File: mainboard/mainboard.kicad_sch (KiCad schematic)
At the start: 54 parts, among them J1 Servo, J2 Buzzer, J4 Button Interface, J5 Power, J6 Release Button, J7 Extra Pins, Q1 BSS138, SW1 SW_Push, U1 RP2040, U2 W25Q128JVS, U3 RV-3028-C7, U4 ITR9608-F, Y1 Crystal_ABM8

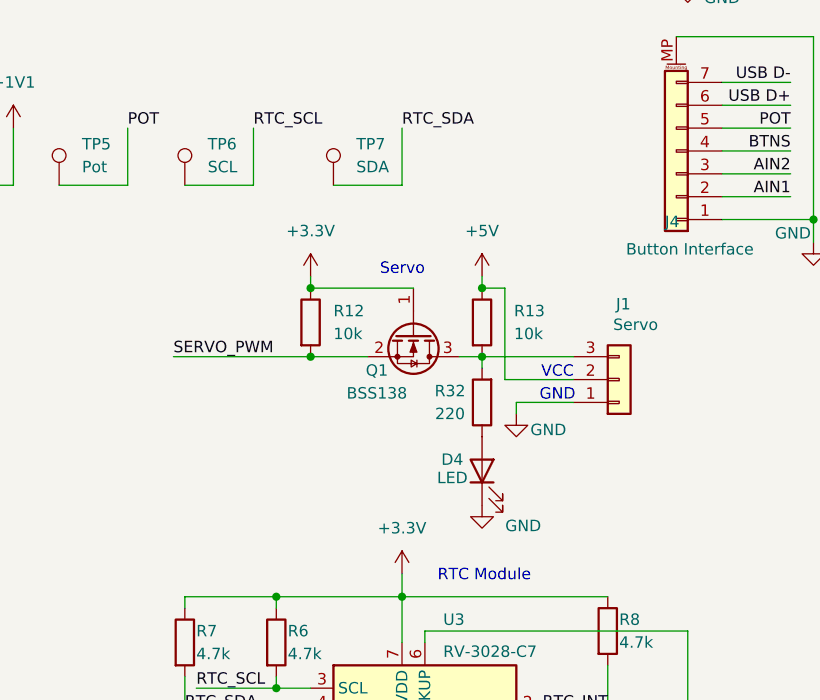
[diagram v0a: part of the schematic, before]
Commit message: Minor fixes
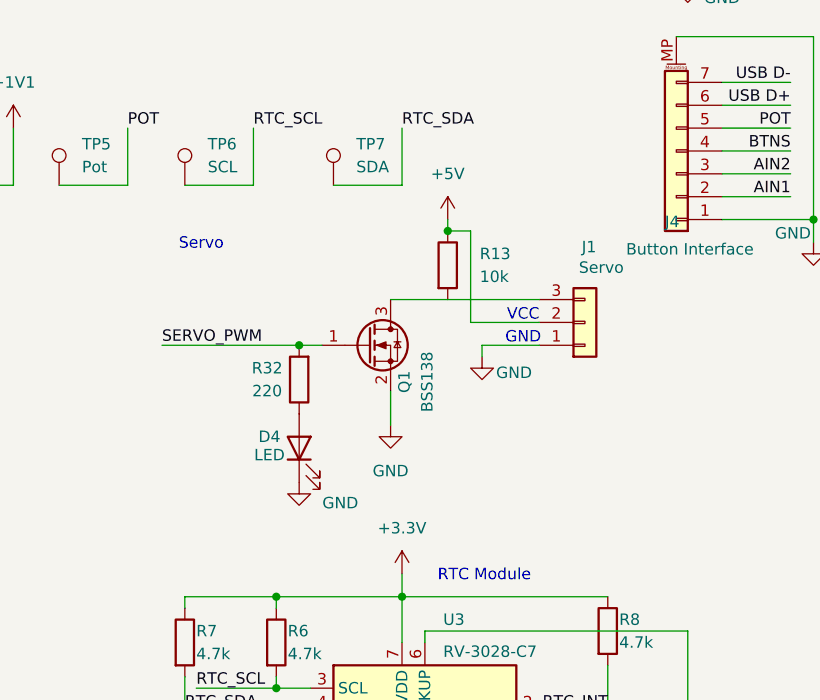
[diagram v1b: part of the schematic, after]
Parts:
- removed R12: 10k, Resistor_SMD:R_0402_1005Metric, symbol Device:R
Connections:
- net +3.3V: no longer Q1.1 (G)
- net GND: now also Q1.2 (S)
- net SERVO_PWM: now also Q1.1 (G), R32.2; no longer Q1.2 (S)
- net at J1.3 (Pin_3), Q1.3 (D): no longer R13.2, R32.2
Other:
- moved on the sheet: D4, J1, Q1, R13, R32
